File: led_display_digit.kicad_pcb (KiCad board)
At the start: 2 copper layers, 51.2 x 22.2 mm, 118 parts, among them J1 Conn_01x05, J2 Conn_01x07, Q1 2N7002, Q2 2N7002, Q3 2N7002, Q4 2N7002

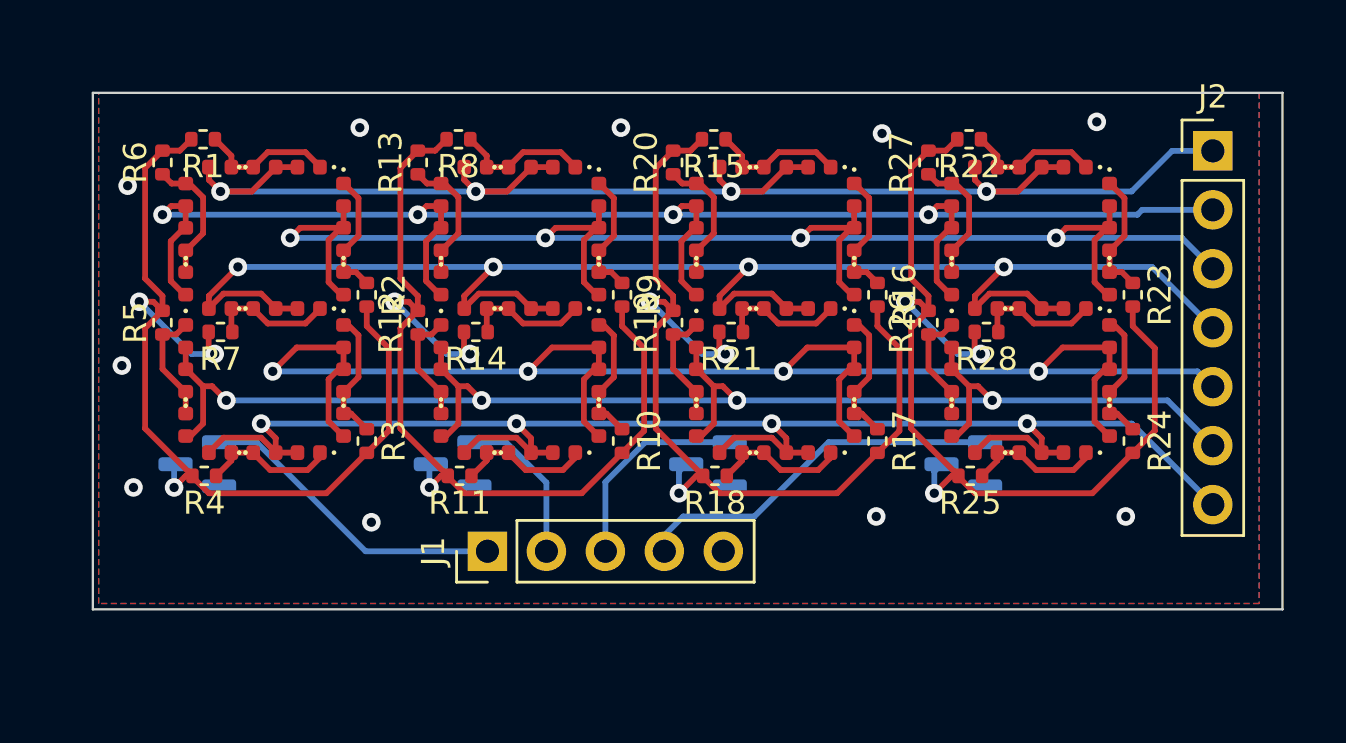
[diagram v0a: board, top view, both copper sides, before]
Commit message: little design changes
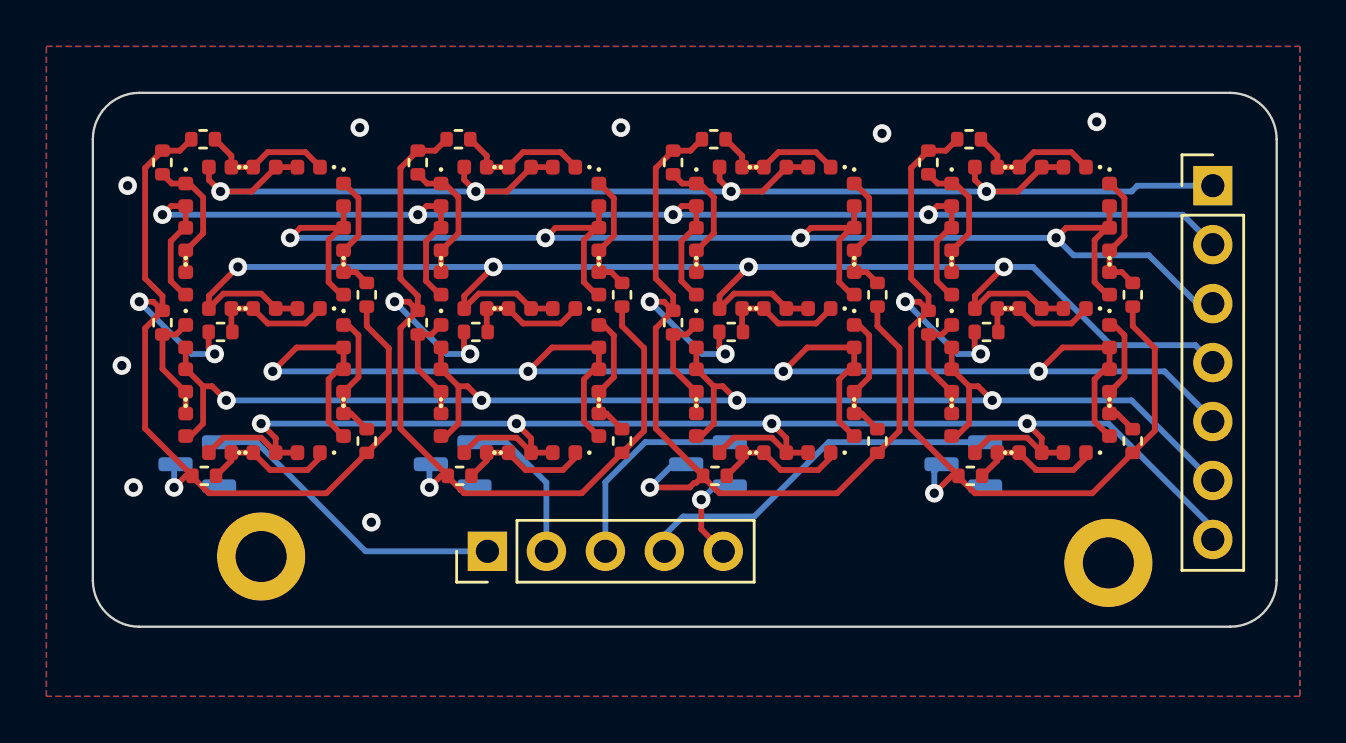
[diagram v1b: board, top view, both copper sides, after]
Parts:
- added H1: MHole, MountingHole:MountingHole_2.2mm_M2_DIN965_Pad, F.Cu at (77.2, 75.0)
- added H2: MHole, MountingHole:MountingHole_2.2mm_M2_DIN965_Pad, F.Cu at (113.8, 75.2)
- added REF**: OSHW-Logo2_9.8x8mm_SilkScreen, Symbol:OSHW-Logo2_9.8x8mm_SilkScreen, B.Cu at (80.8, 64.2)
- added REF**: KiCad-Logo2_6mm_SilkScreen, Symbol:KiCad-Logo2_6mm_SilkScreen, B.Cu at (100.8, 61.8)
- moved J2 1.50 mm to (118.2, 59.0)
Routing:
- net GND: track 0.00 -> 4.08 mm, vias 10 -> 9
- net Net-(Q3-Pad3): track 42.0 -> 43.8 mm
- net Seg_D: track 66.0 -> 66.9 mm
- net Seg_C: track 72.6 -> 73.3 mm
- net Seg_G: track 69.8 -> 70.4 mm
- net Seg_B: track 68.1 -> 68.8 mm
- net Seg_E: track 66.6 -> 67.2 mm
- net Seg_A: track 63.5 -> 62.9 mm
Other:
- board size 51.2 x 22.2 mm -> 51 x 23 mm
- board text added: "A"
- board text added: "B"
- board text added: "C"
- board text added: "D"
- board text added: "D1"
- board text added: "D2"
- board text added: "D3"
- board text added: "D4"
- board text added: "E"
- board text added: "F"
- board text added: "G"
- board text added: "GND"
- board text added: "GitHub"
- board text added: "darioGg3"
